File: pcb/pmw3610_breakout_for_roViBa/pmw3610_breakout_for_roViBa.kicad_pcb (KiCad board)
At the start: 2 copper layers, 22 x 23.5 mm, 13 parts, among them J1 Conn_01x08, U1 MCP1700T-1802E/TT, U2 PMW3610

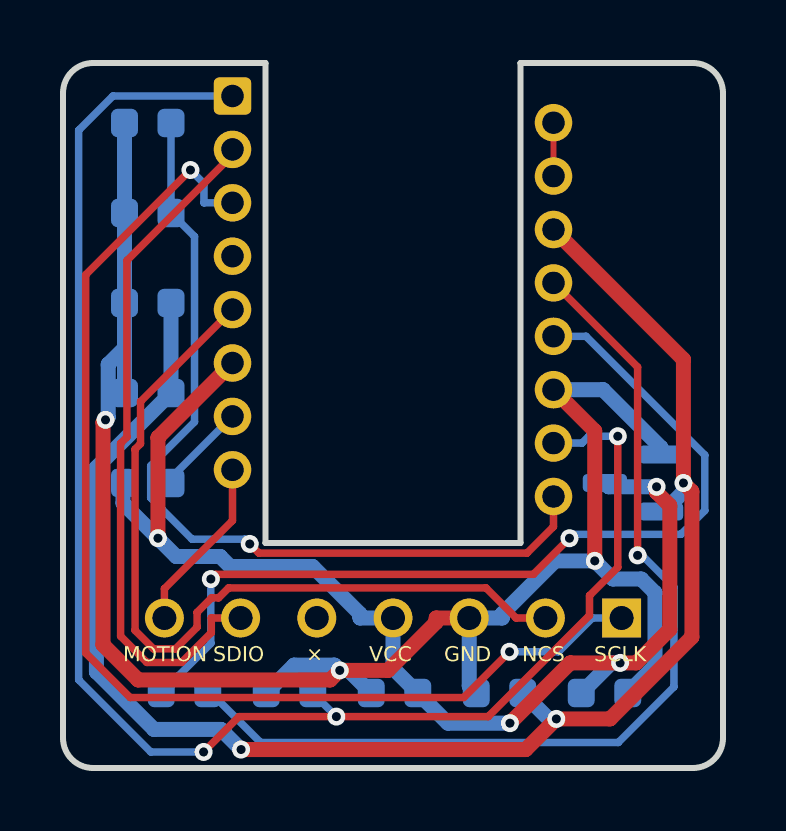
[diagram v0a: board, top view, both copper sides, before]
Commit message: Redo pmw3610 sensor board
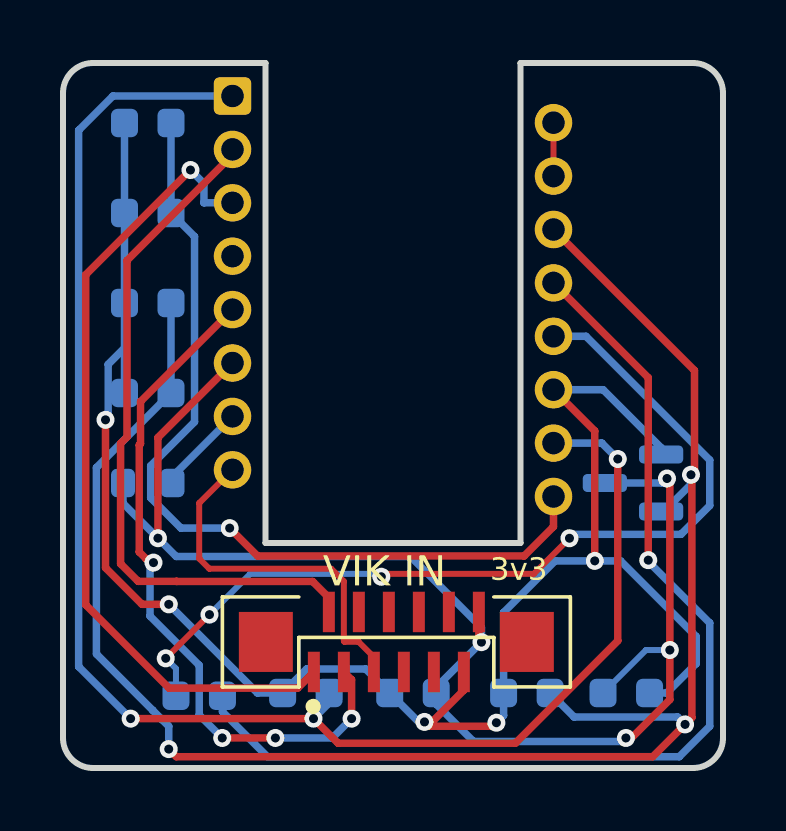
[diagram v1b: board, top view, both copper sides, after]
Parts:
- removed J1: Conn_01x08, roBa:pmw3610_connector_b
- added J2: vik-module-connector, vik:vik-module-connector-vertical, F.Cu at (136.1, 99.3)
- C5: value 100n (X7R) -> 100n (X7R)
- C6: value 10u (X7R) -> 10u (X7R)
- C7: value 10n (X7R) -> 10n (X7R)
- moved C2 0.91 mm to (140.5, 101.0)
- moved C1 0.73 mm to (143.8, 101.0)
- moved C3 0.61 mm to (136.7, 101.0)
- moved C4 0.55 mm to (133.1, 101.0)
- moved C5 0.50 mm to (129.5, 101.1)
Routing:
- net SCLK: track 39.4 -> 27.1 mm, vias 2 -> 1
- net VCC: track 39.6 -> 46.7 mm, vias 4 -> 5
- net MOTION: track 5.88 -> 12.6 mm
- net +1V9: track 54.1 -> 59.9 mm
- net NCS: track 27.5 -> 23.1 mm, vias 0 -> 4
- net Net-(U2-CN): track 32.2 -> 35.0 mm
- net GND: track 61.8 -> 60.6 mm, vias 3 -> 5
- net Net-(U2-CP): track 30.4 -> 30.1 mm, vias 2 -> 4
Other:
- board text removed: "GND"
- board text removed: "MOTION"
- board text removed: "NCS"
- board text removed: "SCLK"
- board text removed: "SDIO"
- board text removed: "VCC"
- board text removed: "×"
